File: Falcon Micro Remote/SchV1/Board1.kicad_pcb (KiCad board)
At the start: 2 copper layers, 37 parts, among them J51 Conn_01x03_Male, SW31 SW_Push, SW51 SW_Push, SW61 SW_Push, SW62 SW_Push, SW63 SW_Push, SW64 SW_Push, SW71 SW_Push, SW72 SW_Push, SW73 SW_Push, SW74 SW_Push, SW75 SW_Push, SW76 SW_Push, U1 AMS1117-3.3, U2 ESP32-WROOM-32

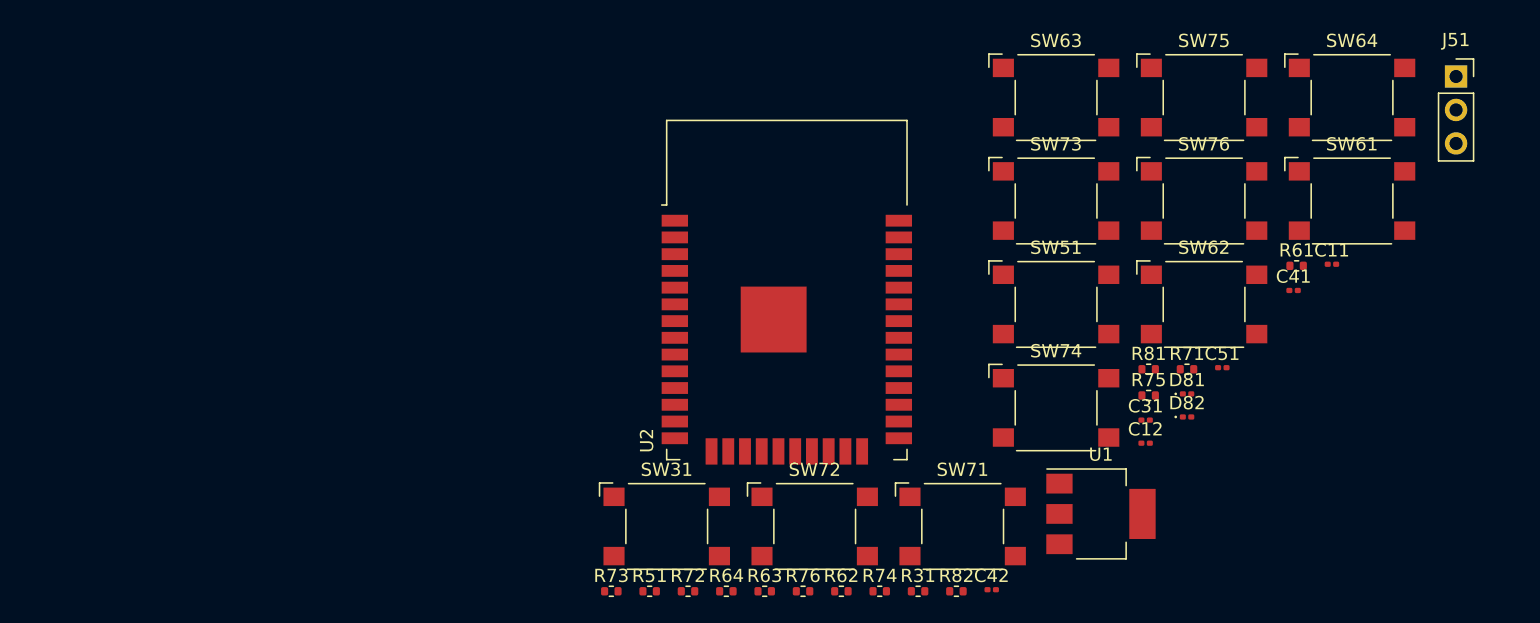
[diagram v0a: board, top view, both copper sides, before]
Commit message: Made modifications to sch and brd files
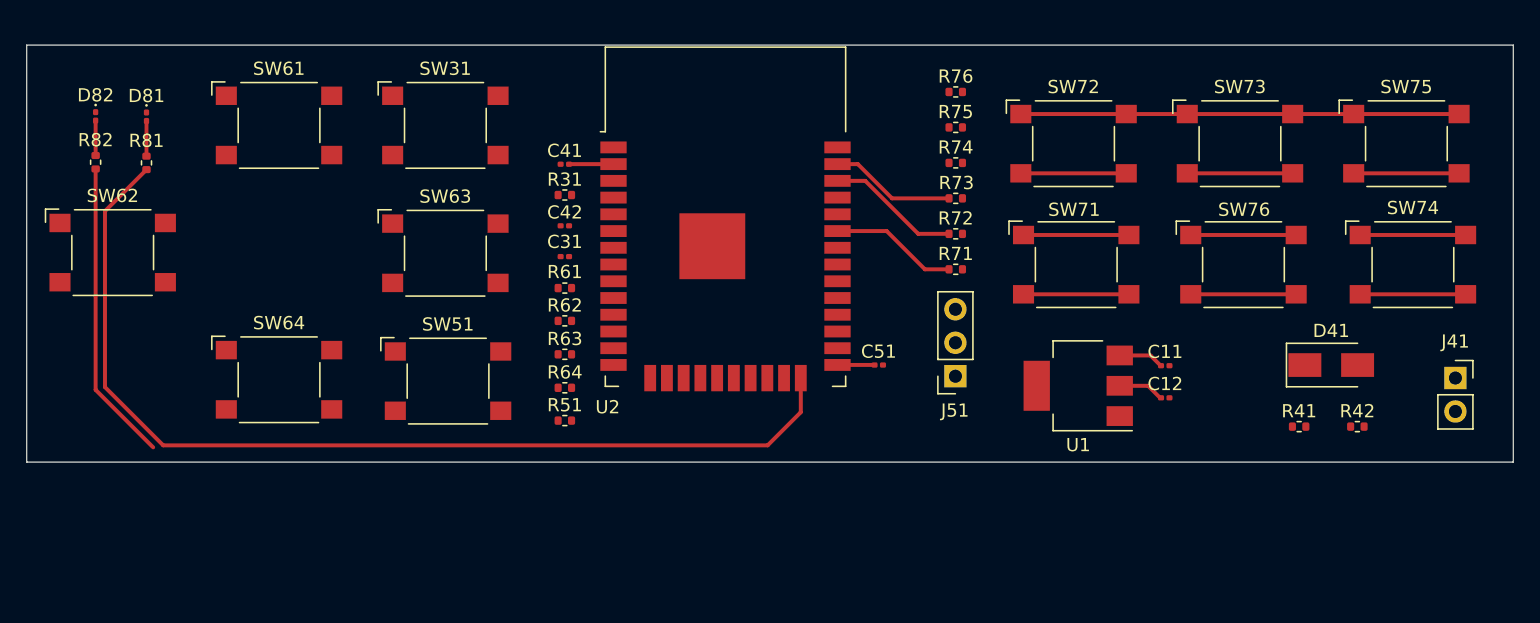
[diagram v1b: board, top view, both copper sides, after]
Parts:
- added D41: SS34, Diode_SMD:D_SMA, F.Cu at (175.2, 84.1)
- added J41: Conn_01x02_Male, Connector_PinSocket_2.54mm:PinSocket_1x02_P2.54mm_Vertical, F.Cu at (184.6, 85.1)
- added R41: 20K, Resistor_SMD:R_0402_1005Metric, F.Cu at (172.8, 88.7)
- added R42: 1K, Resistor_SMD:R_0402_1005Metric, F.Cu at (177.2, 88.7)
- R81, R82: value 200 -> 205
- moved D82 85.9 mm to (81.4, 65.2), turned to -90 degrees
- moved SW64 84.2 mm to (95.4, 85.2)
- moved SW62 82.9 mm to (82.7, 75.5)
- moved D81 81.7 mm to (85.3, 65.2), turned to -90 degrees
- moved SW61 81.6 mm to (95.4, 65.9)
- moved R81 77.7 mm to (85.3, 68.7), turned to 90 degrees
- moved R82 73.0 mm to (81.4, 68.7), turned to 90 degrees
- moved C41 56.1 mm to (117.0, 68.8), turned to 180 degrees
- moved R61 55.6 mm to (117.0, 78.2), turned to 180 degrees
- moved SW63 47.8 mm to (108.0, 75.6)
- moved SW51 46.5 mm to (108.2, 85.3)
- moved C31 45.8 mm to (117.0, 75.8)
- moved J51 44.3 mm to (146.7, 84.9), turned to 180 degrees
- moved C42 42.6 mm to (117.0, 73.5)
- moved R31 40.3 mm to (117.0, 71.2)
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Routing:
- net LED1: track 0.00 -> 76.1 mm
- net 3.3V: track 0.00 -> 64.1 mm
- net LED2: track 0.00 -> 22.9 mm
- net R2: track 0.00 -> 18.1 mm
- net R1: track 0.00 -> 17.7 mm
- net RT: track 0.00 -> 17.5 mm
- net LT: track 0.00 -> 8.00 mm
- net L2: track 0.00 -> 8.00 mm
- net L1: track 0.00 -> 8.00 mm
- net VIN: track 0.00 -> 3.34 mm
- net BOOT: track 0.00 -> 2.82 mm
- net Net-(D81-Pad2): track 0.00 -> 2.68 mm
- net Net-(D82-Pad2): track 0.00 -> 2.65 mm
- net TX: track 0.00 -> 0.78 mm
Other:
- board outline added: 112.8 x 31.6 mm
